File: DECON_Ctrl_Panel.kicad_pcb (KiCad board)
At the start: 2 copper layers, 174 x 105.4 mm, 272 parts, among them J1 Conn_01x02, J10 Conn_01x04, J11 Conn_01x06, J12 Conn_01x06, J13 Conn_01x04, J18 Conn_01x04, J2 Conn_01x06, J3 Conn_01x06, J4 Conn_01x06, J5 FLASH, J6 Conn_01x06, J7 Conn_01x05, J8 Conn_01x06, J9 Conn_01x06, K1 G5NB, K10 G5NB, K11 G5NB, K12 G5NB, K13 G5NB, K14 G5NB, K15 G5NB, K16 G5NB, K17 G5NB, K2 G5NB, K3 G5NB, K4 G5NB, K5 G5NB, K6 G5NB, K7 G5NB, K8 G5NB, K9 G5NB, Q1 MMBT2222A, Q10 MMBT2222A, Q11 MMBT2222A, Q12 MMBT2222A, Q13 MMBT2222A, Q14 MMBT2222A, Q15 MMBT2222A, Q16 MMBT2222A, Q2 MMBT2222A, Q3 MMBT2222A, Q4 MMBT2222A, Q5 MMBT2222A, Q6 MMBT2222A, Q7 MMBT2222A, Q8 MMBT2222A, Q9 MMBT2222A, SW1 SW_Push, SW2 SW_Push, U1 URB2405YMD-10WR3, U10 LTV-817S, U11 LTV-817S, U12 LTV-817S, U13 LTV-817S, U14 LTV-817S, U15 LTV-817S, U16 LTV-817S, U17 LTV-817S, U18 LTV-817S, U19 LTV-817S, U2 AZ1117-3.3, U21 LTV-817S, U22 LTV-817S, U23 LTV-817S, U24 LTV-817S, U25 LTV-817S, U26 LTV-817S, U27 LTV-817S, U28 LTV-817S, U29 LTV-817S, U3 STM32F401R_B-C_Tx, U30 LTV-817S, U31 LTV-817S, U32 LTV-817S, U33 LTV-817S, U34 LTV-817S, U35 LTV-817S, U36 LTV-817S, U4 LTV-817S, U5 LTV-817S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

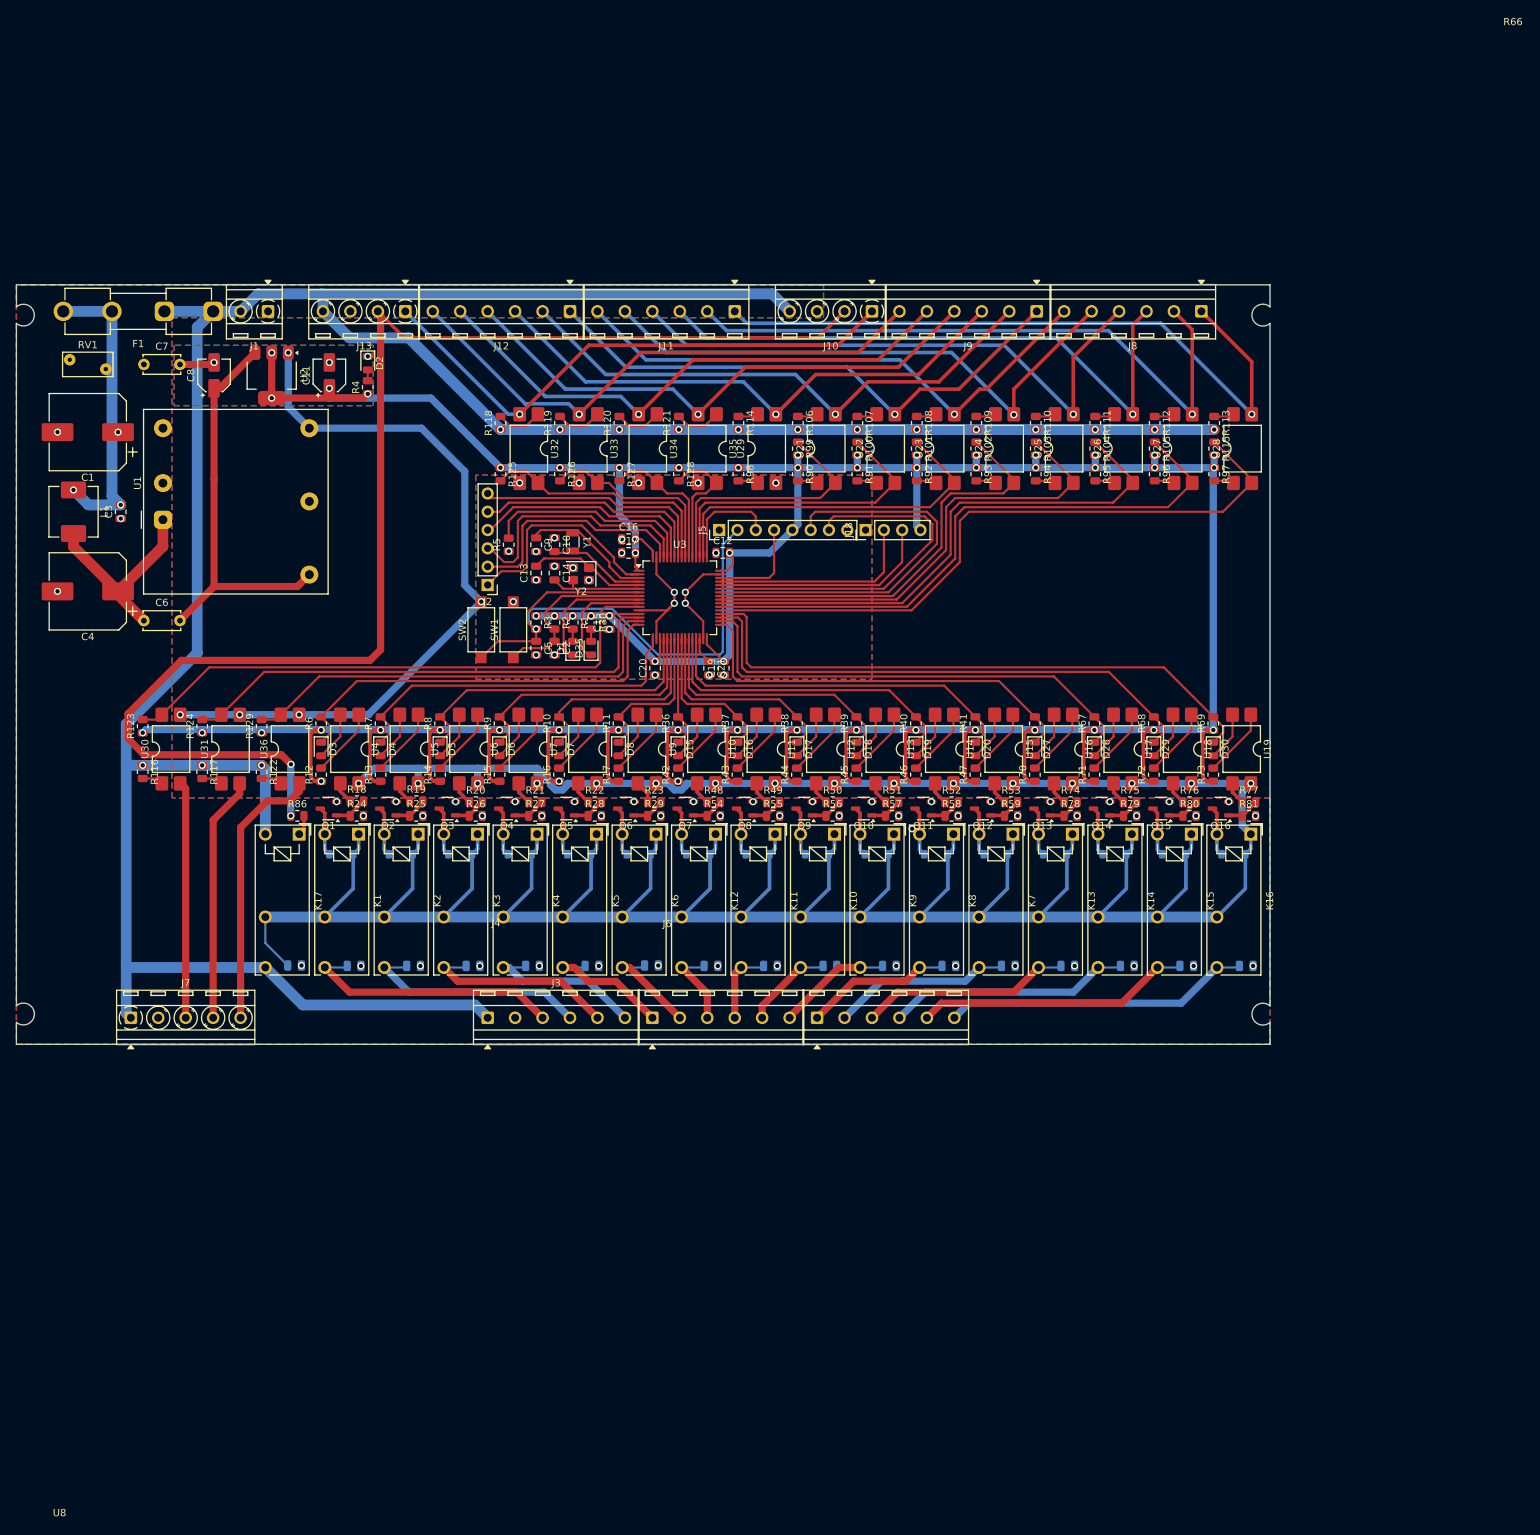
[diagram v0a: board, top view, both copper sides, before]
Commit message: modified:   DECON_Ctrl_Panel.kicad_pcb 	modified:   DECON_Ctrl_Panel.kicad_prl 	modified:   DECON_Ctrl_Panel.kicad_pro 	modified:   decon_mcu.kicad_sch 	new file:   decon_mcu.kicad_sch-bak 	modified:   fp-info-cache 	modified:   relay.kicad_sch 	new file:   relay.kicad_sch-bak
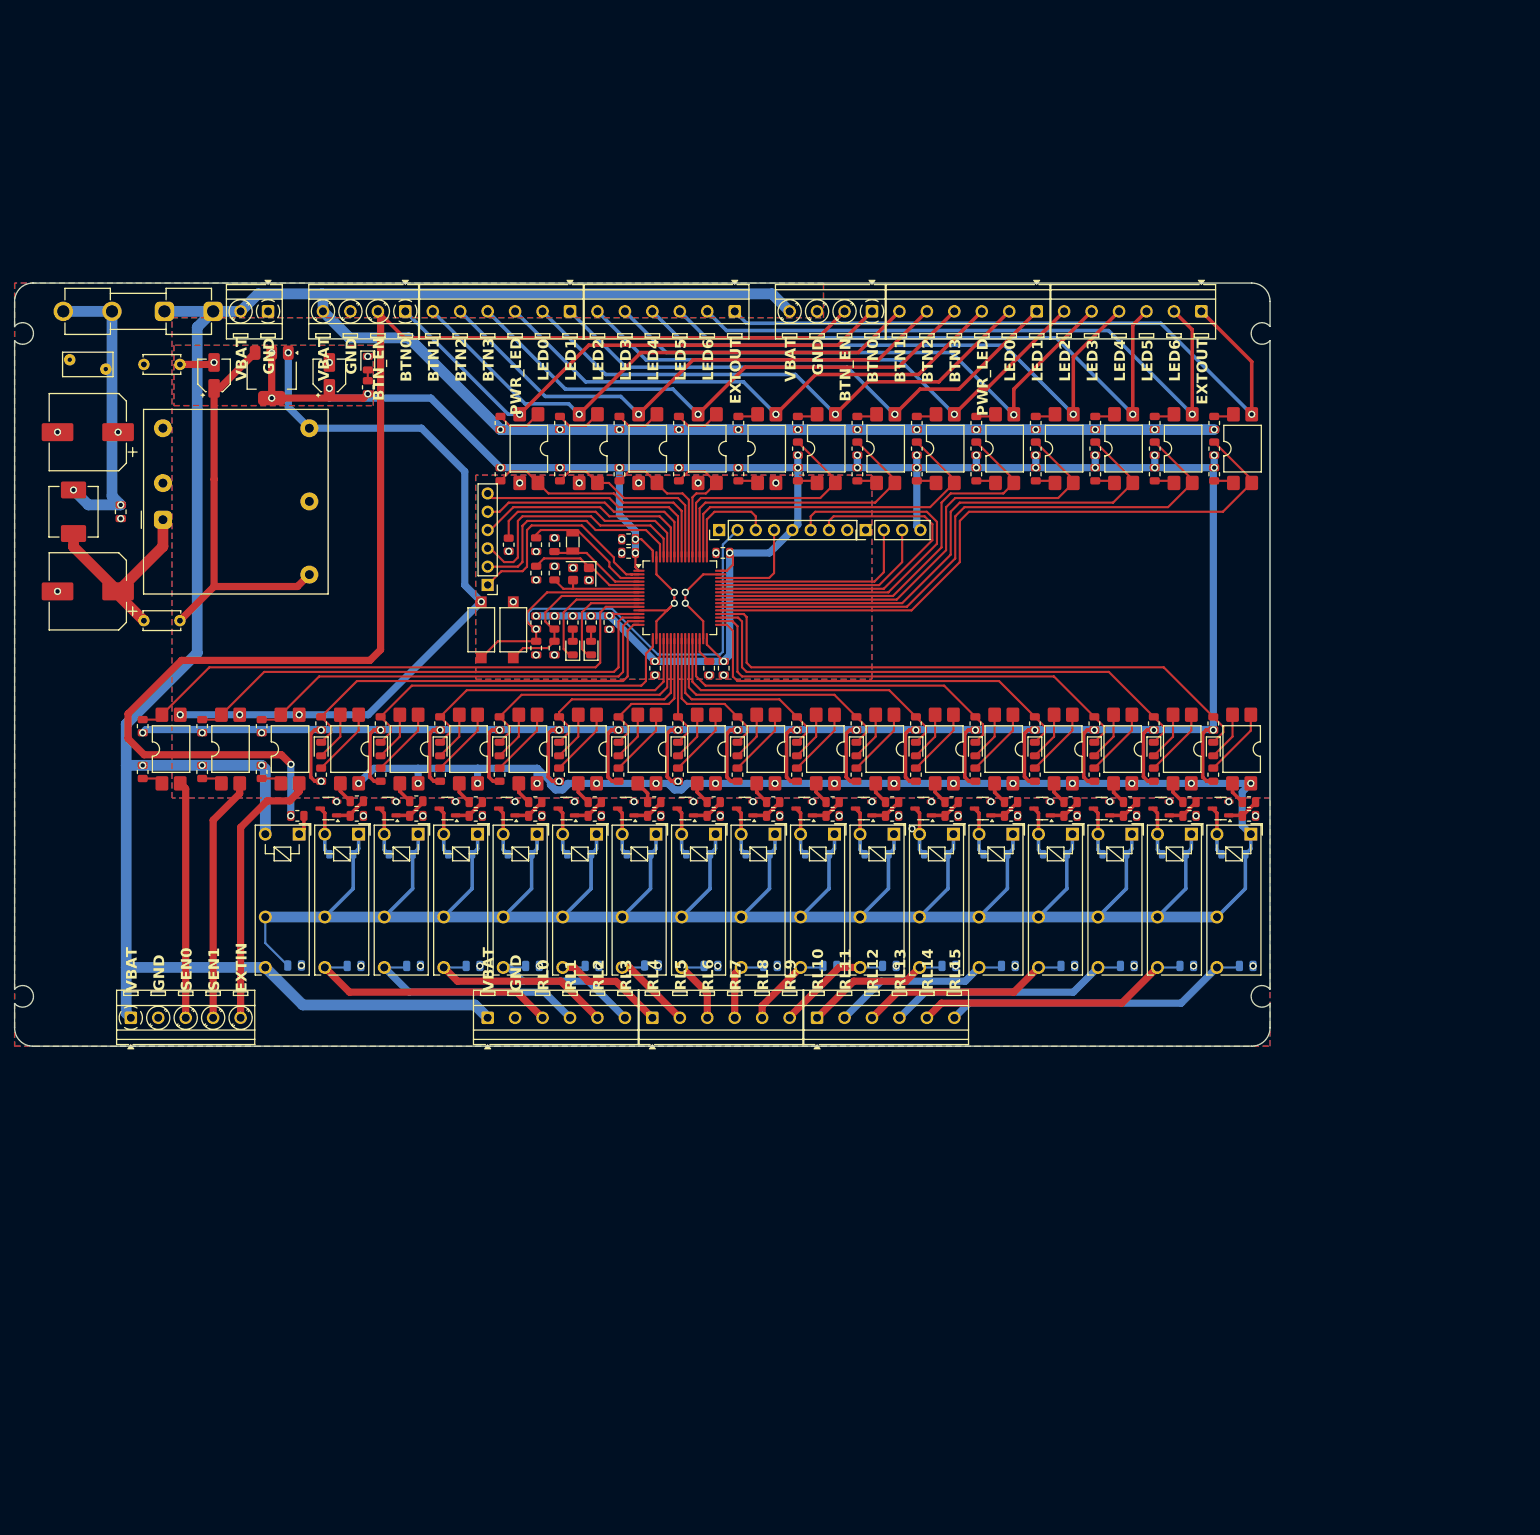
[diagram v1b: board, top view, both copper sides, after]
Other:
- board size 174 x 105.4 mm -> 174.2 x 105.9 mm
- board text added: "BTN0"
- board text added: "BTN1"
- board text added: "BTN2"
- board text added: "BTN3"
- board text added: "BTN_EN"
- board text added: "EXTIN"
- board text added: "EXTOUT"
- board text added: "GND"
- board text added: "LED0"
- board text added: "LED1"
- board text added: "LED2"
- board text added: "LED3"
- board text added: "LED4"
- board text added: "LED5"
- board text added: "LED6"
- board text added: "PWR_LED"
- board text added: "RL0"
- board text added: "RL1"
- board text added: "RL10"
- board text added: "RL11"
- board text added: "RL12"
- board text added: "RL13"
- board text added: "RL14"
- board text added: "RL15"
- board text added: "RL2"
- board text added: "RL3"
- board text added: "RL4"
- board text added: "RL5"
- board text added: "RL6"
- board text added: "RL7"
- board text added: "RL8"
- board text added: "RL9"
- board text added: "SEN0"
- board text added: "SEN1"
- board text added: "VBAT"
